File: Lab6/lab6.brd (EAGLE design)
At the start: 106 x 106 mm, 56 parts, among them J1 ISP, Q1 SI2302CDS, Q2 SI2302CDS, Q3 SI2302CDS, Q4 SI2302CDS, U1 ATMEGA128RFA1, Y1 16MHz

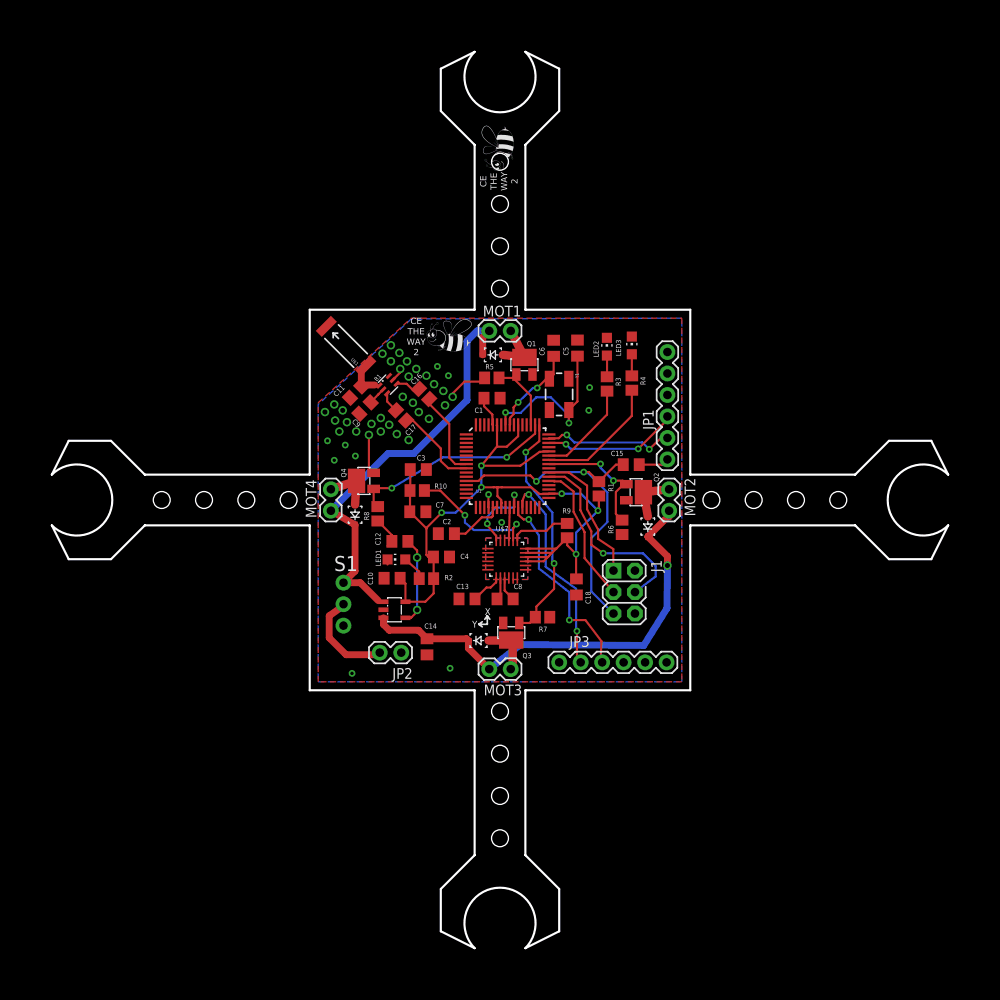
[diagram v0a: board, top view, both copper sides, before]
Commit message: Fixed What Swanson Wanted
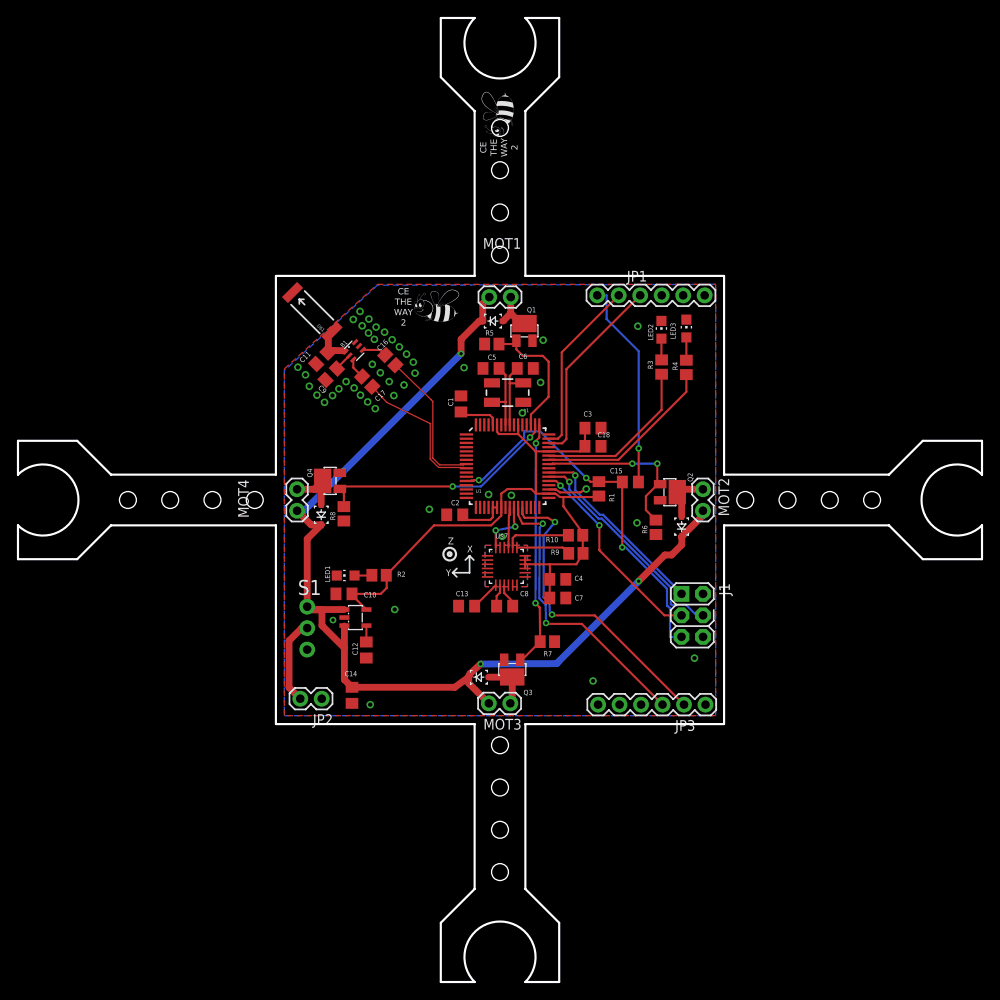
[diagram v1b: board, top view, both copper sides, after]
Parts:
- moved C3 21.2 mm to (11.0, 8.50)
- moved JP1 21.1 mm to (11.5, 24.2), turned to 0 degrees
- moved R10 19.5 mm to (8.94, -4.17), turned to 180 degrees
- moved C7 19.4 mm to (6.83, -11.6)
- moved JP3 18.0 mm to (24.3, -24.2), turned to 180 degrees
- moved C18 16.7 mm to (11.0, 6.35), turned to 0 degrees
- moved C4 14.0 mm to (6.83, -9.39)
- moved C12 13.4 mm to (-15.8, -17.7), turned to 270 degrees
- moved JP2 10.9 mm to (-22.4, -23.5)
- moved C14 10.6 mm to (-17.5, -23.1)
- moved C5 10.5 mm to (-1.06, 15.6), turned to 180 degrees
- moved J1 8.51 mm to (22.7, -13.6)
- moved LED2 6.75 mm to (19.1, 20.1)
- moved LED3 6.75 mm to (22.0, 20.3)
- moved R3 6.75 mm to (19.1, 15.7)
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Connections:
- net RFN renamed RF_N
- net RFP renamed RF_P
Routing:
- net N$3: track 3.59 -> 24.8 mm, vias 0 -> 1
- net VBAT: track 104.7 -> 124.4 mm, vias 1 -> 3
- net 3V: track 101.2 -> 81.6 mm, vias 6 -> 0
- net GND: track 17.4 -> 4.64 mm, vias 43 -> 46
- net TX1: track 24.7 -> 37.0 mm
- net N$5: track 19.9 -> 8.61 mm, vias 2 -> 0
- net RX1: track 23.9 -> 34.5 mm
- net N$2: track 10.4 -> 1.94 mm, vias 2 -> 0
- net PB7: track 11.7 -> 19.8 mm
- net N$30: track 15.7 -> 7.85 mm, vias 2 -> 0
- net PE5: track 8.66 -> 16.0 mm
- net SCK: track 16.8 -> 24.0 mm, vias 0 -> 2
- net RF_P: track 10.3 -> 17.2 mm
- net MISO: track 16.4 -> 23.3 mm, vias 0 -> 1
- net RF_N: track 10.3 -> 17.2 mm
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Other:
- board size 106 x 106 mm -> 114 x 114 mm
- board text added: "Z"
